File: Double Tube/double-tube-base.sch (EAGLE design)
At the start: 5 parts

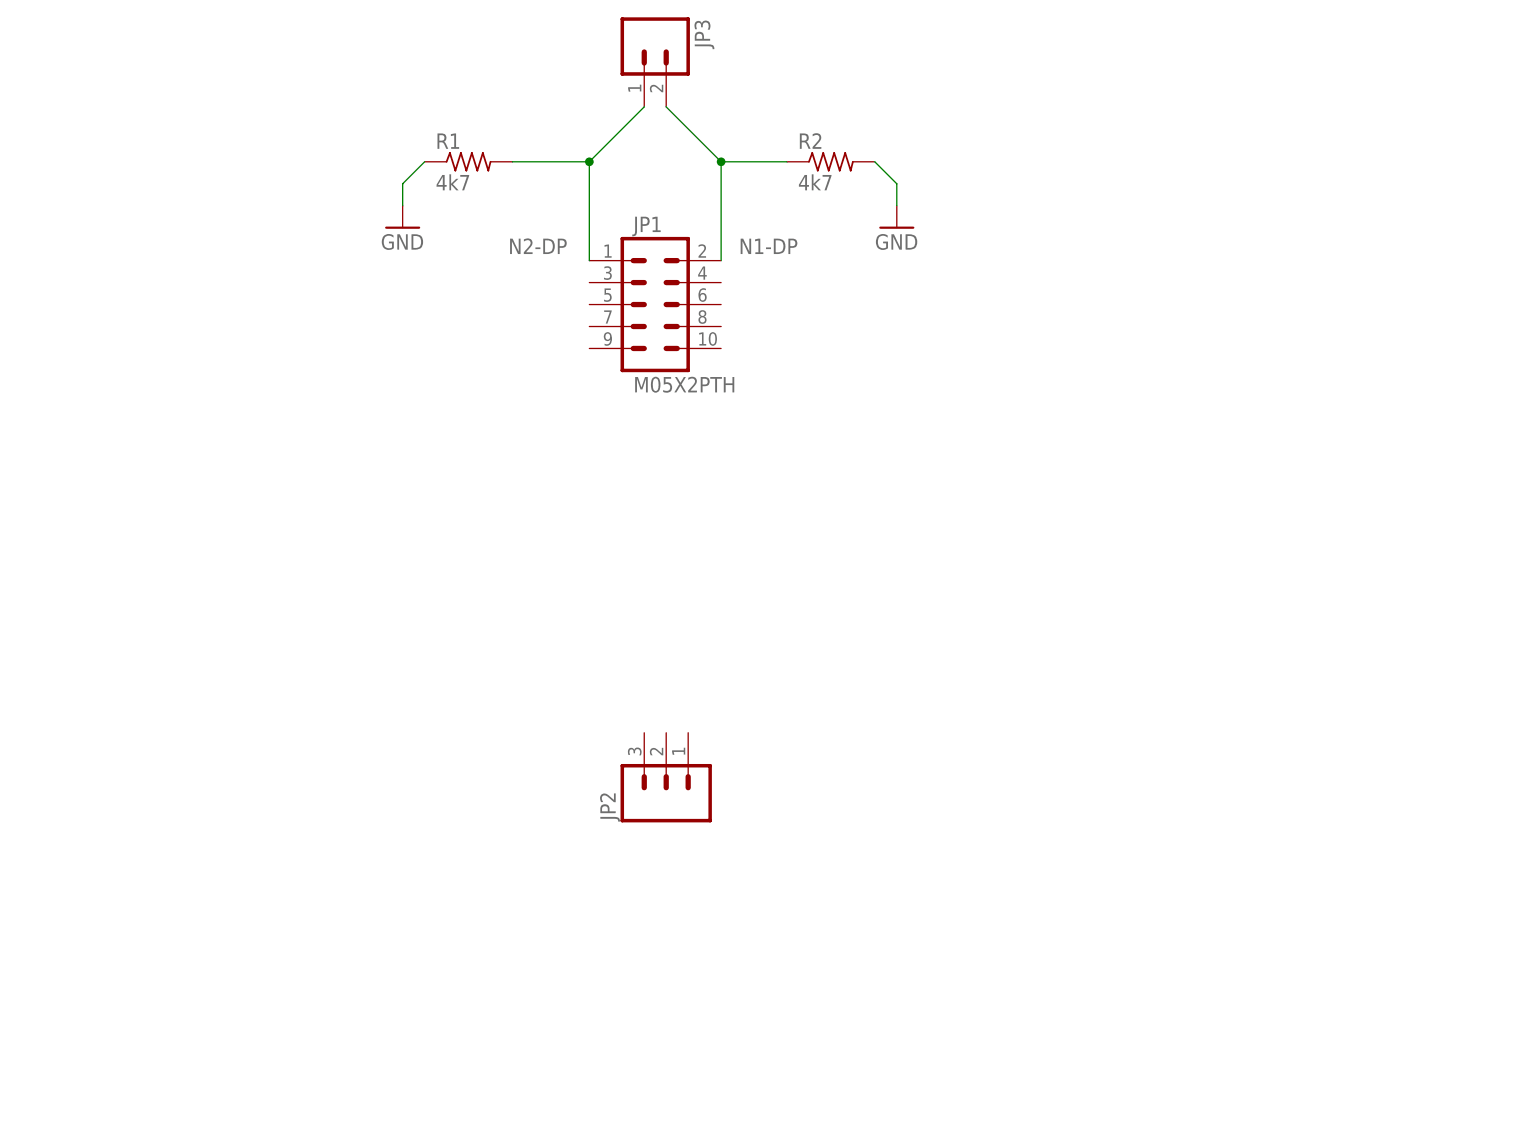
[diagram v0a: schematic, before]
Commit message: Update some files
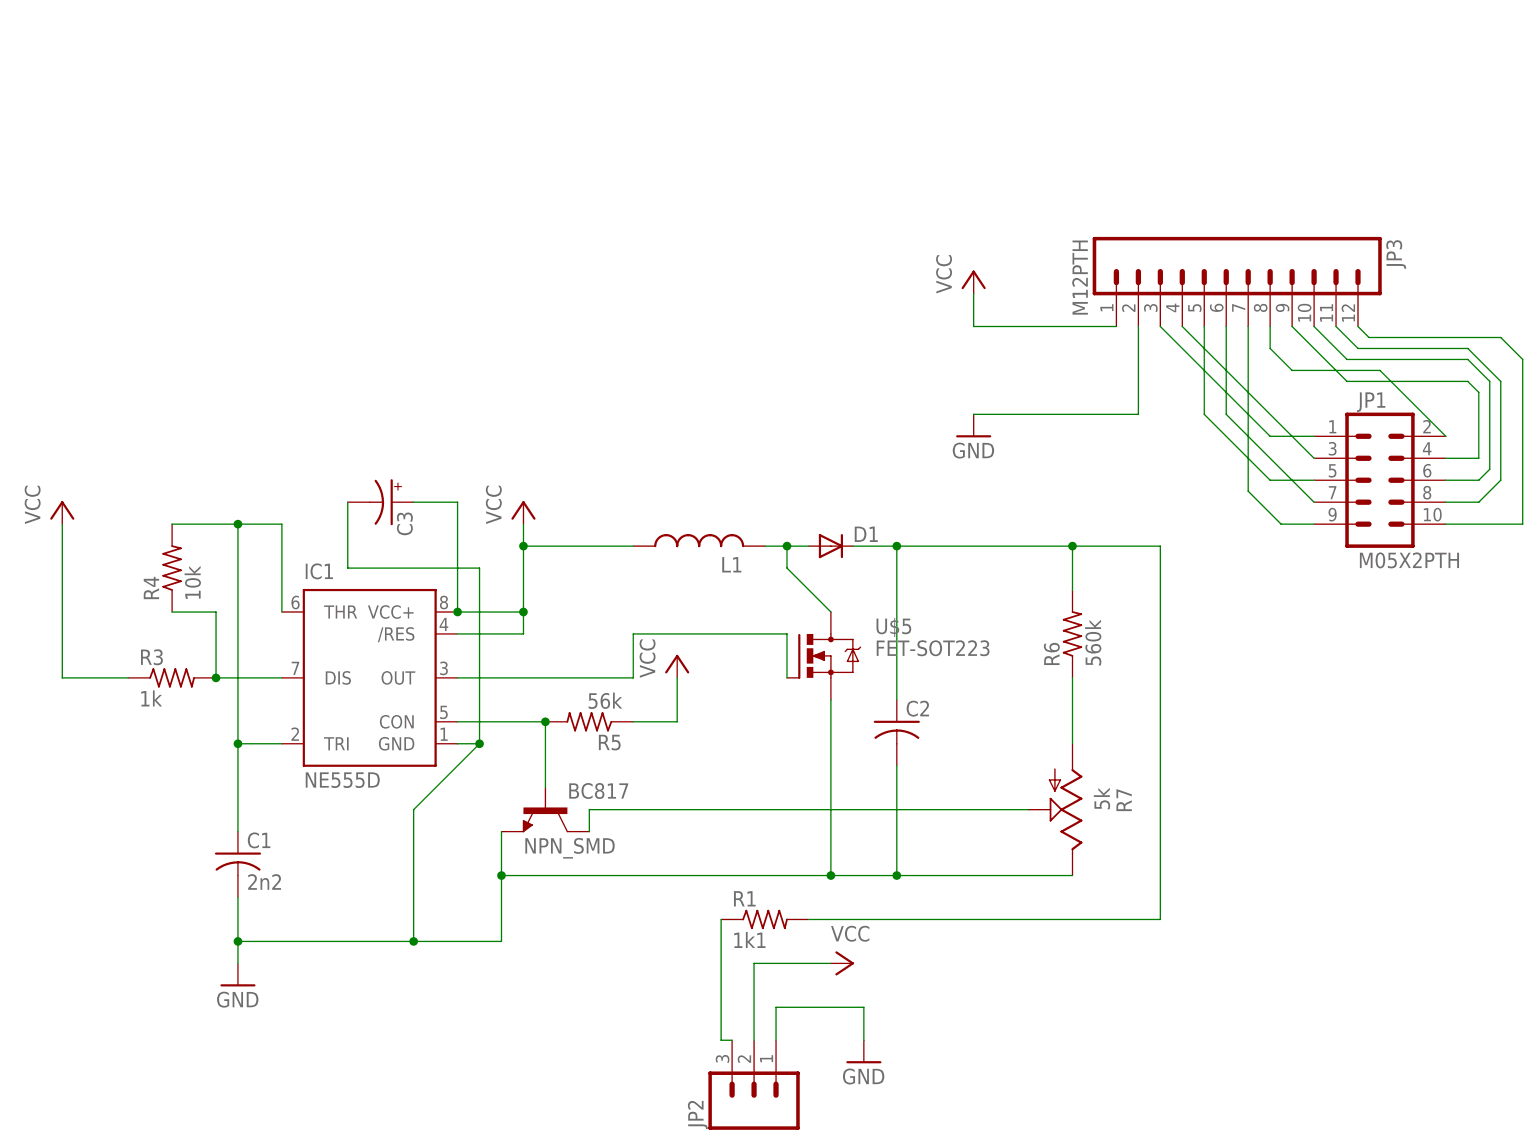
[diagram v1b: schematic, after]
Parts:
- removed R2: 4k7, iStivi - RCLD:RESISTORR0805
- added BC817: NPN_SMD, iStivi - Transistor-FET-reg:NPN_SMD
- added C1: 2n2, iStivi - RCLD:CAPACITORC0603K
- added C2: (no value), iStivi - RCLD:CAPACITORC1812K
- added C3: (no value), iStivi - RCLD:CAPACITOR_POLSMCD
- added D1: (no value), iStivi - RCLD:DIODESMA
- added IC1: NE555D, iStivi - ICs:NE555D
- added L1: (no value), iStivi - RCLD:INDUCTORSMD-10MM
- added R3: 1k, iStivi - RCLD:RESISTORR0603
- added R4: 10k, iStivi - RCLD:RESISTORR0603
- added R5: 56k, iStivi - RCLD:RESISTORR0603
- added R6: 560k, iStivi - RCLD:RESISTORR1206
- added R7: 5k, iStivi - RCLD:TRIM_POTEVM2N
- added U$5: FET-SOT223, iStivi - Transistor-FET-reg:FET-SOT223
- JP3: value (none) -> M12PTH; device iStivi - Header-Connector:M02PTH -> iStivi - Header-Connector:M12PTH
- R1: value 4k7 -> 1k1; device iStivi - RCLD:RESISTORR0805 -> iStivi - RCLD:RESISTORR1206
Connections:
- removed net N1-DP: JP1.2, JP3.2, R2.1
- removed net N2-DP: JP1.1, JP3.1, R1.2
- new net N$1: IC1.DIS, R3.2, R4.1
- new net N$11: JP1.1, JP3.3
- new net N$12: JP1.3, JP3.4
- new net N$13: JP1.5, JP3.5
- new net N$14: JP1.7, JP3.6
- new net N$15: JP1.9, JP3.7
- new net N$16: JP1.2, JP3.8
- new net N$17: JP1.4, JP3.9
- new net N$18: JP1.6, JP3.10
- new net N$19: JP1.8, JP3.11
- new net N$2: C1.1, IC1.THR, IC1.TRI, R4.2
- new net N$20: JP1.10, JP3.12
- new net N$3: BC817.B, IC1.CON, R5.2
- new net N$4: D1.A, L1.2, U$5.D
- new net N$5: C2.1, D1.C, R1.2, R6.2
- new net N$6: BC817.C, R7.S
- new net N$7: R6.1, R7.A
- new net N$8: IC1.OUT, U$5.G
- new net N$9: JP2.3, R1.1
- new net VCC: C3.+, IC1./RES, IC1.VCC+, JP2.2, JP3.1, L1.1, R3.1, R5.1
- net GND: now also BC817.E, C1.2, C2.2, C3.-, IC1.GND, JP2.1, JP3.2, R7.E, U$5.S; no longer R1.1, R2.2
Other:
- moved on the sheet: JP1, JP2, R1
